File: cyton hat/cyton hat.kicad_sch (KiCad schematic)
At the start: 13 parts, among them J1 Conn_02x13_Odd_Even, J2 Conn_01x08, J3 Conn_01x04, J4 Conn_01x02, J5 Conn_01x04

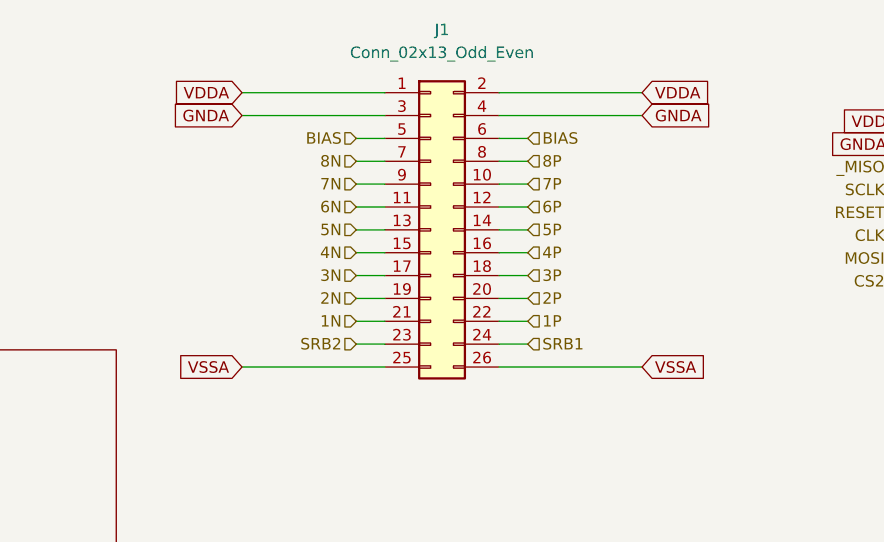
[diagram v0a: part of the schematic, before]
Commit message: finished layout
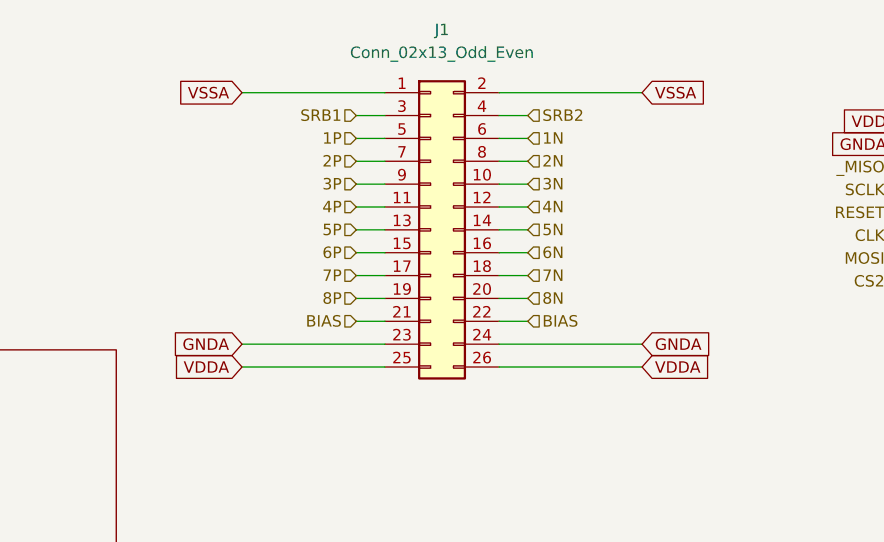
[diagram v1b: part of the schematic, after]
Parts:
- C19, C20, C21, C22, C23, C24, C25, C26: footprint (none) -> Capacitor_SMD:C_0402_1005Metric
- J1: footprint (none) -> Connector_PinHeader_2.54mm:PinHeader_2x13_P2.54mm_Horizontal
- J2: footprint (none) -> Connector_PinSocket_2.54mm:PinSocket_1x08_P2.54mm_Vertical
- J3, J5: footprint (none) -> Connector_PinSocket_2.54mm:PinSocket_1x04_P2.54mm_Vertical
- J4: footprint (none) -> Connector_PinSocket_2.54mm:PinSocket_1x02_P2.54mm_Vertical
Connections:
- net 1N: now also J1.6 (Pin_6); no longer J1.21 (Pin_21)
- net 1P: now also J1.5 (Pin_5); no longer J1.22 (Pin_22)
- net 2N: now also J1.8 (Pin_8); no longer J1.19 (Pin_19)
- net 2P: now also J1.7 (Pin_7); no longer J1.20 (Pin_20)
- net 3N: now also J1.10 (Pin_10); no longer J1.17 (Pin_17)
- net 3P: now also J1.9 (Pin_9); no longer J1.18 (Pin_18)
- net 4N: now also J1.12 (Pin_12); no longer J1.15 (Pin_15)
- net 4P: now also J1.11 (Pin_11); no longer J1.16 (Pin_16)
- net 5N: now also J1.14 (Pin_14); no longer J1.13 (Pin_13)
- net 5P: now also J1.13 (Pin_13); no longer J1.14 (Pin_14)
- net 6N: now also J1.16 (Pin_16); no longer J1.11 (Pin_11)
- net 6P: now also J1.15 (Pin_15); no longer J1.12 (Pin_12)
- net 7N: now also J1.18 (Pin_18); no longer J1.9 (Pin_9)
- net 7P: now also J1.17 (Pin_17); no longer J1.10 (Pin_10)
- net 8N: now also J1.20 (Pin_20); no longer J1.7 (Pin_7)
- net 8P: now also J1.19 (Pin_19); no longer J1.8 (Pin_8)
- net BIAS: now also J1.21 (Pin_21), J1.22 (Pin_22); no longer J1.5 (Pin_5), J1.6 (Pin_6)
- net GNDA: now also J1.23 (Pin_23), J1.24 (Pin_24); no longer J1.3 (Pin_3), J1.4 (Pin_4)
- net SRB1: now also J1.3 (Pin_3); no longer J1.24 (Pin_24)
- net SRB2: now also J1.4 (Pin_4); no longer J1.23 (Pin_23)
- net VDDA: now also J1.25 (Pin_25), J1.26 (Pin_26); no longer J1.1 (Pin_1), J1.2 (Pin_2)
- net VSSA: now also J1.1 (Pin_1), J1.2 (Pin_2); no longer J1.25 (Pin_25), J1.26 (Pin_26)
